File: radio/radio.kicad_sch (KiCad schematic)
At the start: 18 parts, among them J1 Conn_01x04, J2 ESP32_LEFT, J3 ESP32_RIGHT, J4 FM_SPEAKERS, J5 RADIO_MIC, J6 ANTENNA_VHF, J7 BATTERY_18650, J8 POWER_SWITCH, SW1 ROTARY_ENCODER, SW2 SW_Push, SW3 SW_Push, SW4 SW_Push, U2 SA828-VHF, U3 RDA5807M-FM, U4 PAM8403-FM-AMP, U5 TP4056_CHARGER, U6 5V_BOOST, U7 3V3_REGULATOR

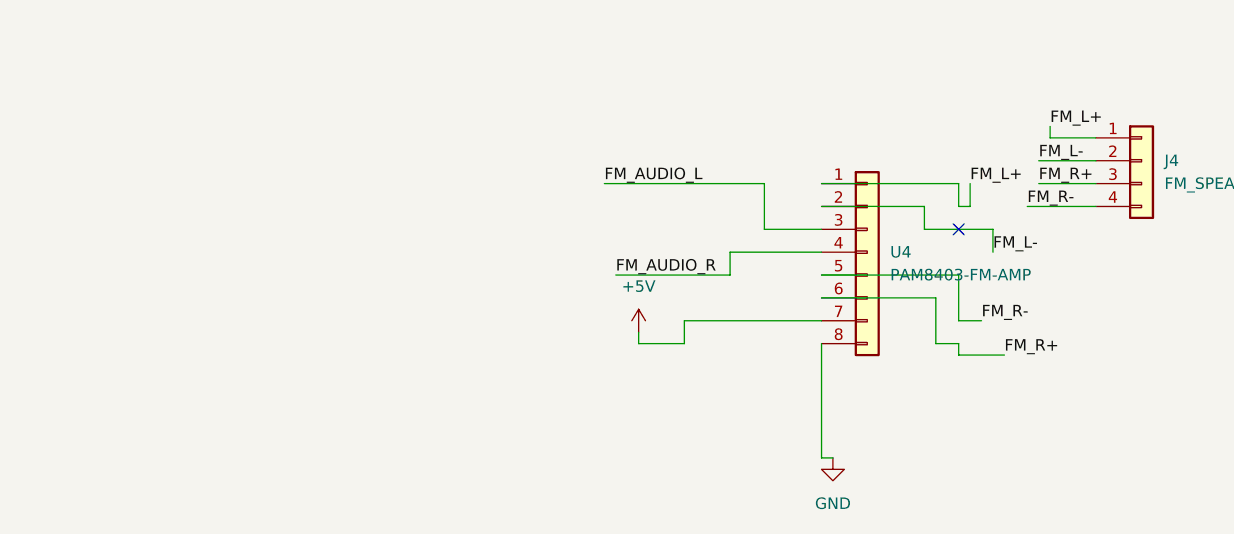
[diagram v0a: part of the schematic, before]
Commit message: pcb_v1
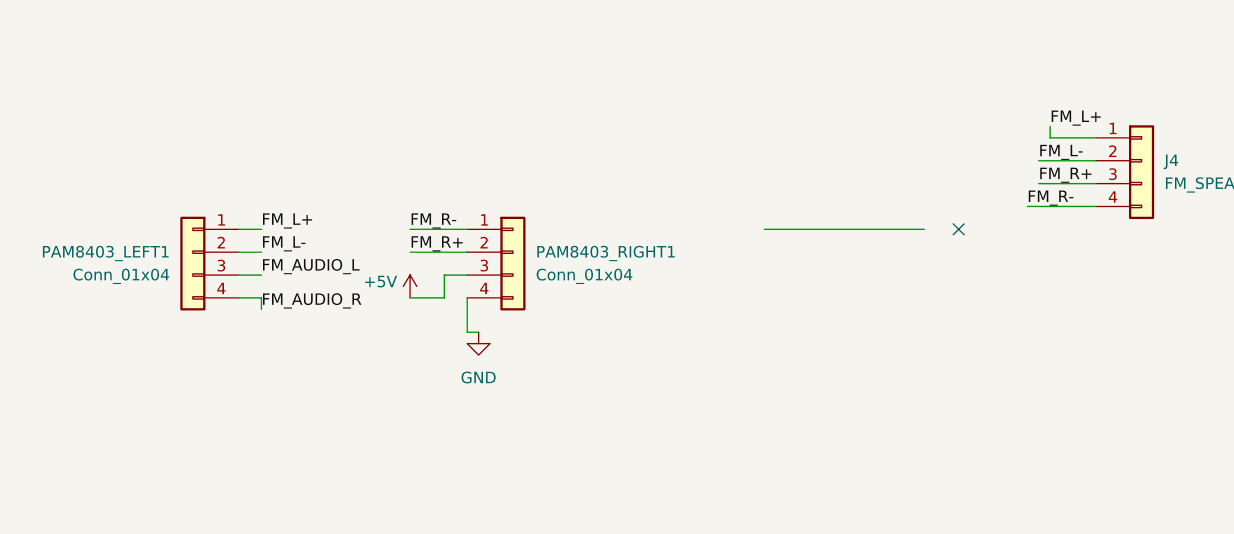
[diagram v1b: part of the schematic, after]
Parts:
- removed U4: PAM8403-FM-AMP, symbol Connector_Generic:Conn_01x08
- added PAM8403_LEFT1, PAM8403_RIGHT1: Conn_01x04, Connector_PinHeader_2.54mm:PinHeader_1x04_P2.54mm_Vertical, symbol Connector_Generic:Conn_01x04
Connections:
- net +5V: now also PAM8403_RIGHT1.3 (Pin_3)
- net FM_AUDIO_L: now also PAM8403_LEFT1.3 (Pin_3)
- net FM_AUDIO_R: now also PAM8403_LEFT1.4 (Pin_4)
- net FM_L+: now also PAM8403_LEFT1.1 (Pin_1)
- net FM_L-: now also PAM8403_LEFT1.2 (Pin_2)
- net FM_R+: now also PAM8403_RIGHT1.2 (Pin_2)
- net FM_R-: now also PAM8403_RIGHT1.1 (Pin_1)
- net GND: now also PAM8403_RIGHT1.4 (Pin_4)
